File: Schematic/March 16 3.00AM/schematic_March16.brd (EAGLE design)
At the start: 167.3 x 150.8 mm, 314 parts, among them CON1 UBC05V128-B0C04D, IC1 FT232RL, IC10 TL084D, IC13 7805TV, IC3 TL084D, IC4 TL084D, IC5 TL084D, IC6 TL084D, IC7 TL084D, IC8 TL084D, IC9 TL084D, Q2 BC557, T1 BC547, T2 BC547, U1 TMS320F28069_PN_80, U10 REF2030AIDDCR, U2 TLV5610_PW_20, U3 REF2030AIDDCR, U4 REF2030AIDDCR, U5 TS12A44514DR, U6 TS12A44514DR, U7 TPS7333QD, U8 REF2030AIDDCR, U9 MAX395CWG+

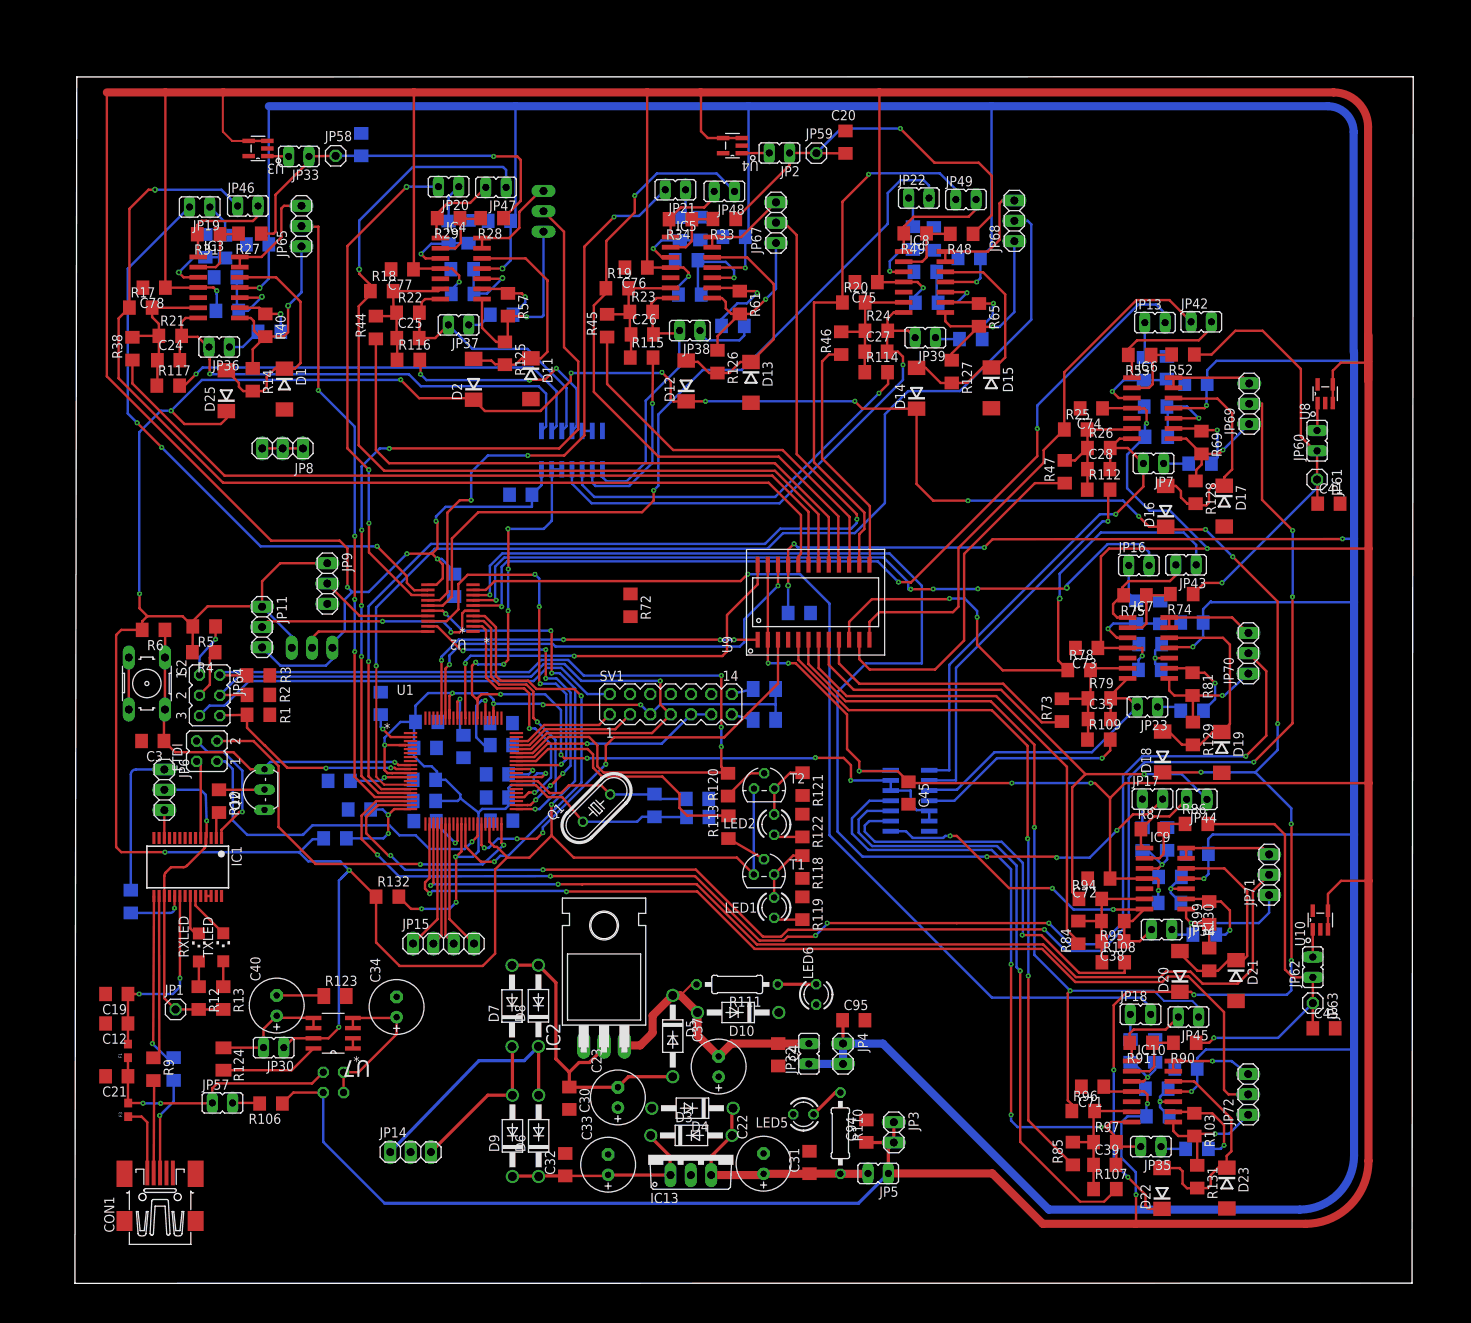
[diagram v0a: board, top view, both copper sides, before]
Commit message: Grounding complete
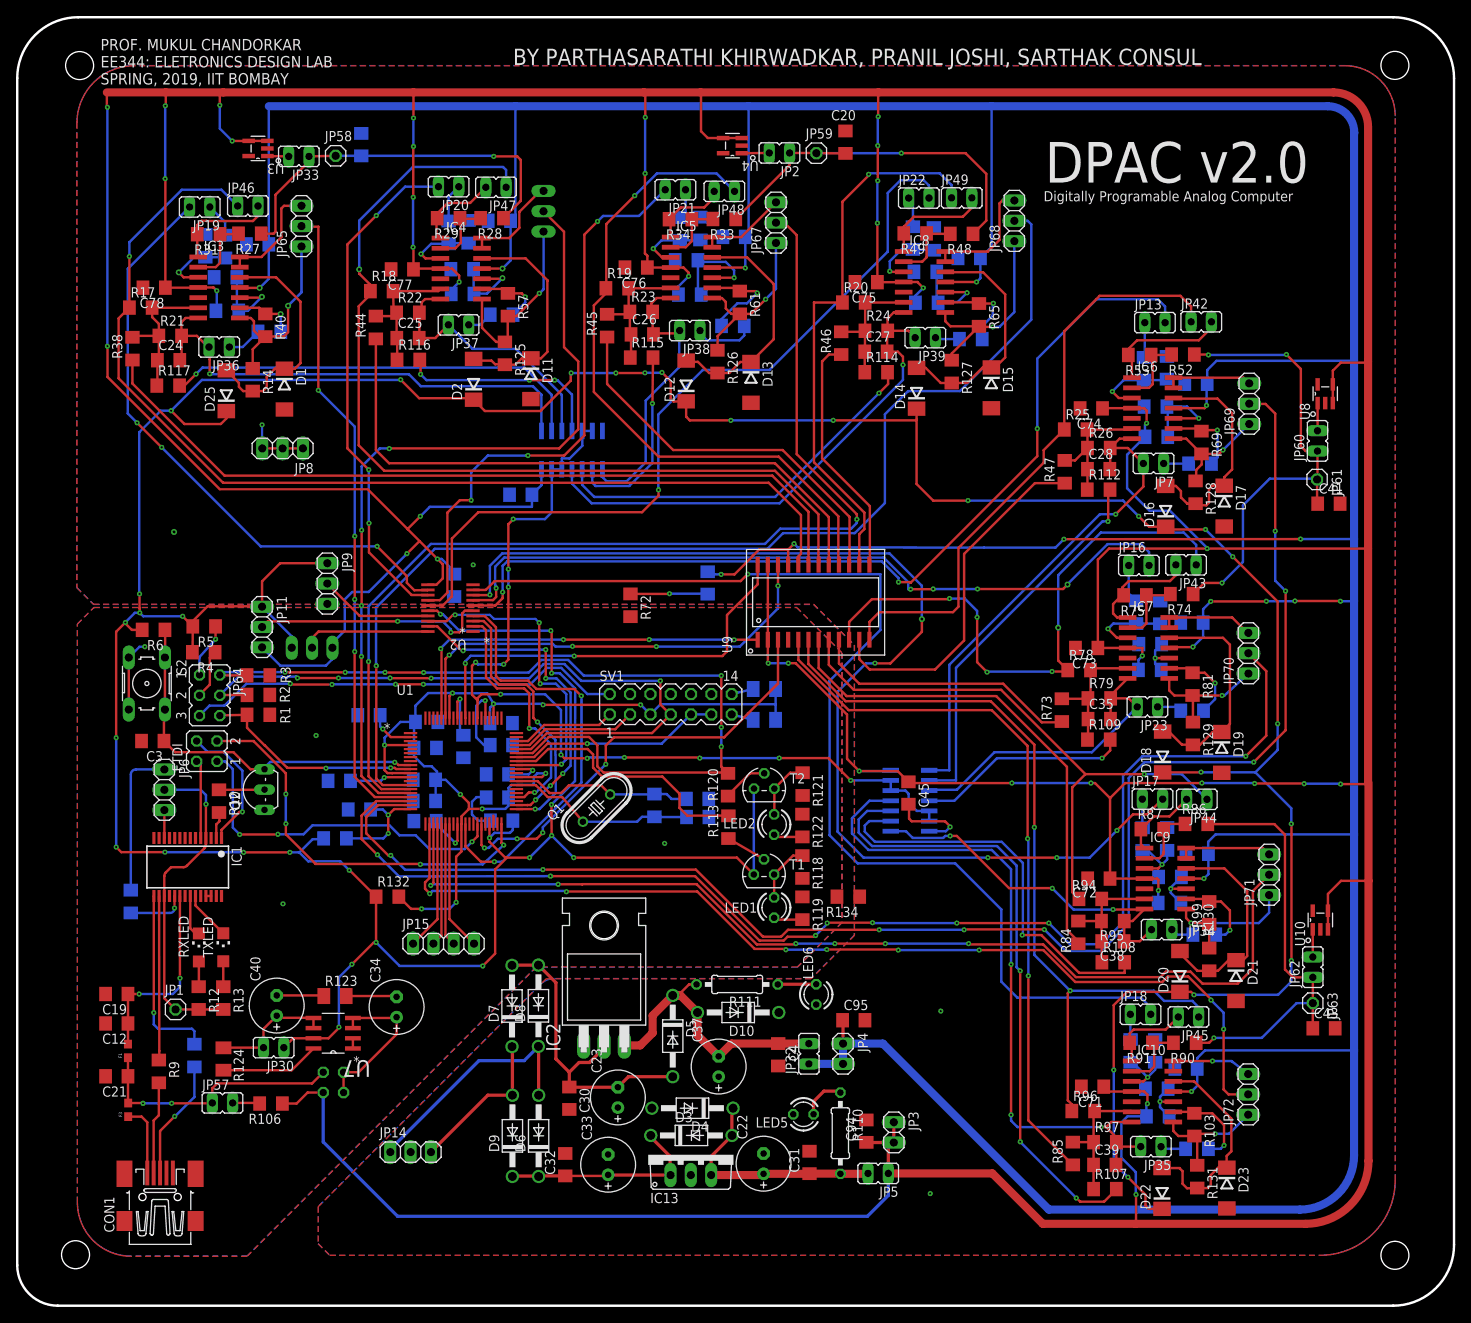
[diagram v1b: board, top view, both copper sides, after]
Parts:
- added R134: 0, rcl:R1206
- moved C42 12.1 mm to (83.6, -14.6), turned to 270 degrees
- moved R8 3.09 mm to (19.5, -73.7)
- moved C5 2.08 mm to (41.3, -31.1), turned to 0 degrees
- moved R9 0.74 mm to (15.0, -75.7)
- moved JP49 0.57 mm to (115.4, 33.5)
- moved JP60 0.06 mm to (159.9, 3.15)
- turned C29 to 0 degrees
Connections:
- removed net SV1-2: JP14.2
- net AGND: now also JP14.2, R134.1
- net GND: now also R134.2
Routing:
- net AGND: track 5.08 -> 28.0 mm, vias 0 -> 7
- net DACO8: track 125.8 -> 142.2 mm
- net GND: track 8.42 -> 24.7 mm, vias 0 -> 4
- net LDACBAR: track 50.2 -> 40.9 mm
- net VDDIO: track 138.7 -> 131.9 mm, vias 9 -> 10
- net -5V: track 638.4 -> 643.4 mm, vias 12 -> 16
- net INT_CONTROL: track 113.7 -> 118.3 mm, vias 10 -> 12
- net INTINP5: track 69.6 -> 74.2 mm
- net DACO5: track 112.7 -> 116.8 mm
- net +1.5V2: track 51.9 -> 48.5 mm
- net N$12: track 12.3 -> 15.1 mm
- net INTSWITCH2: track 28.8 -> 26.4 mm
- net INTINP1: track 135.8 -> 133.4 mm
- net DACO7: track 146.4 -> 144.0 mm, vias 4 -> 6
- net +3V3: track 585.5 -> 583.2 mm, vias 25 -> 41
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- added copper zone on layer 1, net AGND
- added copper zone on layer 16, net AGND
- added copper zone on layer 1, net GND
- added copper zone on layer 16, net GND
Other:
- board size 167.3 x 150.8 mm -> 179.6 x 161.1 mm
- board text added: "BY PARTHASARATHI KHIRWADKAR, PRANIL JOSHI, SARTHAK CONSUL"
- board text added: "DPAC v2.0"
- board text added: "Digitally Programable Analog Computer"
- board text added: "PROF. MUKUL CHANDORKAR EE344: ELETRONICS DESIGN LAB SPRING, 2019, IIT BOMBAY"
